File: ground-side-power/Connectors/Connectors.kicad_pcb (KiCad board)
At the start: 2 copper layers, 11 parts, among them J15 To Router, J16 To RLCS, J17 To DAQ Laptop, J18 Conn_01x02_Female, J19 Conn_01x02_Female, J20 To Ethernet, J21 To 5V M12, J22 To DAQ, J23 Extra M12, J24 Extra M12, J25 Extra M12

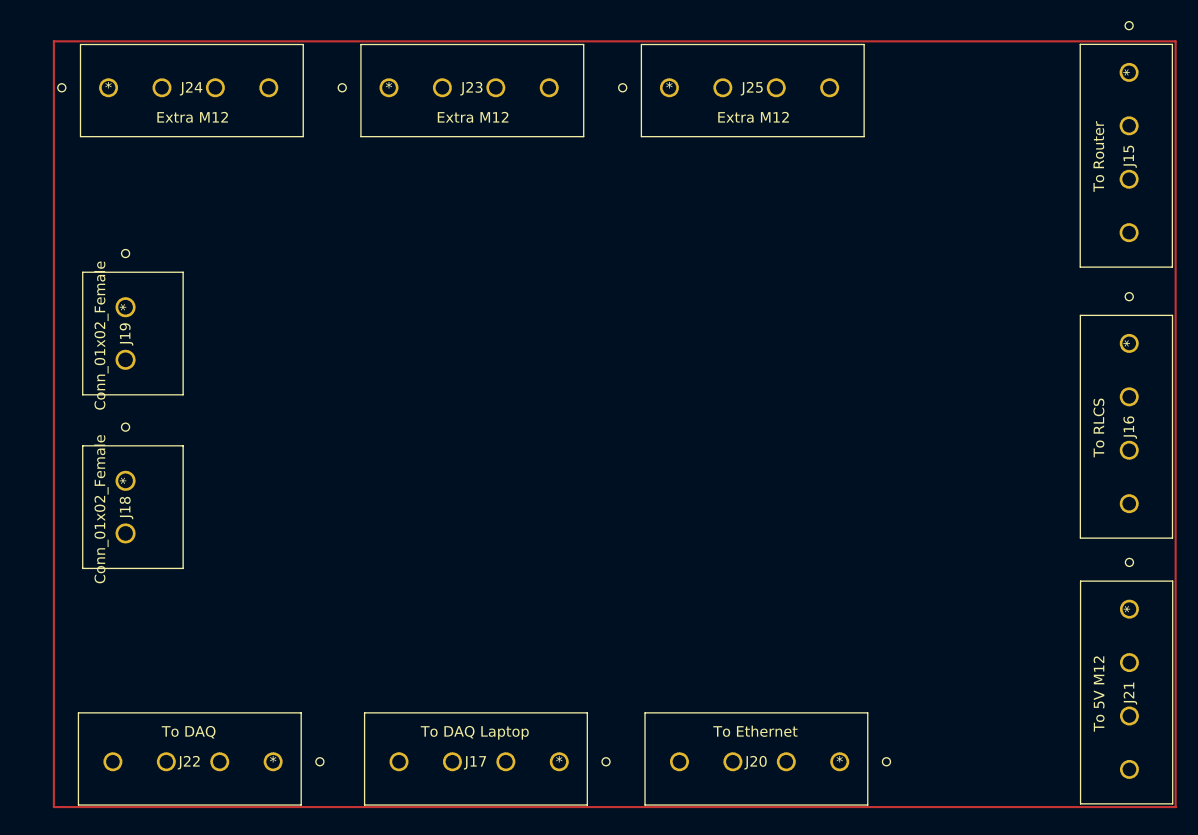
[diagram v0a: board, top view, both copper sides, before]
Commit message: PCB Layout First Draft
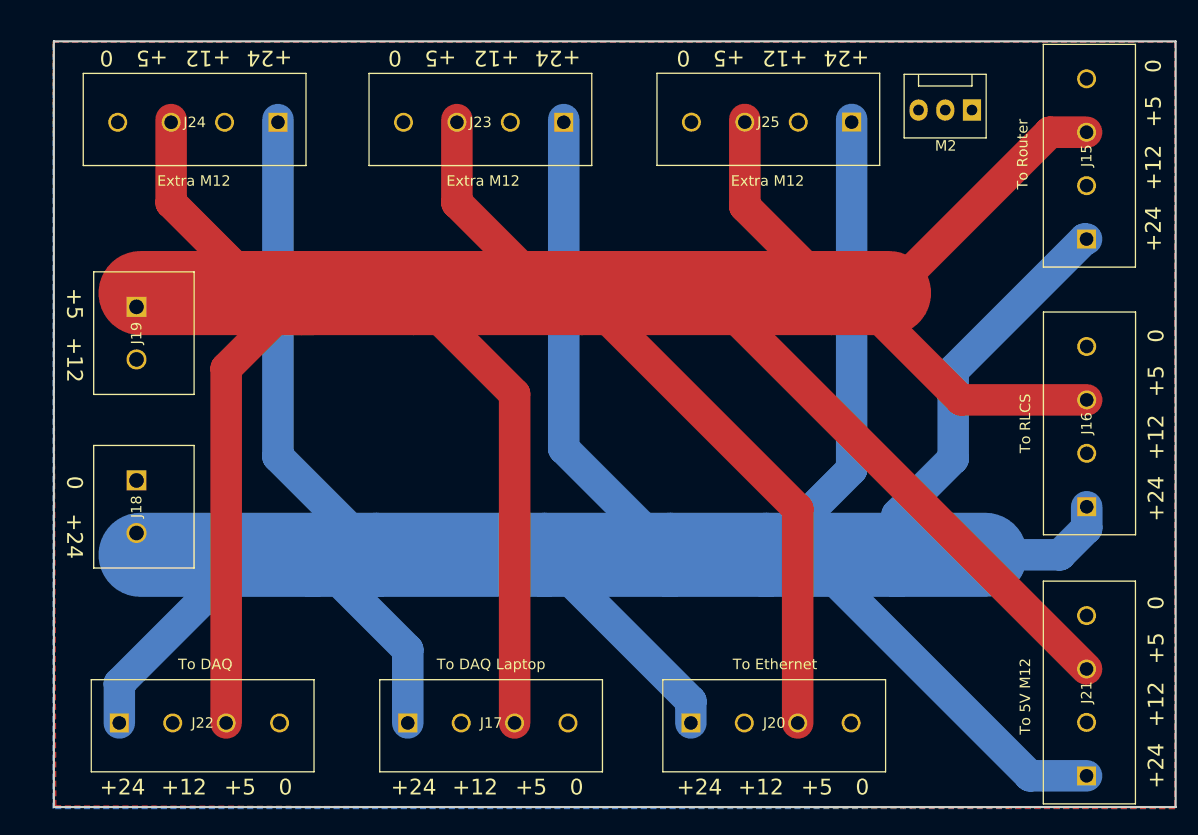
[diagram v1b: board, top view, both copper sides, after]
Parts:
- added M2: Fan_PC_Chassis, Connector:FanPinHeader_1x03_P2.54mm_Vertical, F.Cu at (178.6, 70.5)
- moved J25 17.6 mm to (167.1, 71.6), turned to 180 degrees
- moved J23 16.9 mm to (139.8, 71.6), turned to 180 degrees
- moved J24 16.4 mm to (112.6, 71.6), turned to 180 degrees
- moved J21 16.4 mm to (189.5, 133.8), turned to 90 degrees
- moved J15 16.4 mm to (189.5, 82.7), turned to 90 degrees
- moved J16 16.1 mm to (189.5, 108.2), turned to 90 degrees
- moved J22 15.1 mm to (97.5, 128.8), turned to 0 degrees
- moved J17 14.9 mm to (124.9, 128.8), turned to 0 degrees
- moved J20 14.6 mm to (151.8, 128.8), turned to 0 degrees
- moved J18 1.04 mm to (99.1, 105.7)
- moved J19 1.04 mm to (99.1, 89.2)
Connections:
- J15 pad 1: (no net) -> +24V
- J15 pad 2: (no net) -> +12V
- J15 pad 3: (no net) -> +5V
- J15 pad 4: (no net) -> GND
- J16 pad 1: (no net) -> +24V
- J16 pad 2: (no net) -> +12V
- J16 pad 3: (no net) -> +5V
- J16 pad 4: (no net) -> GND
- J17 pad 1: (no net) -> +24V
- J17 pad 2: (no net) -> +12V
- J17 pad 3: (no net) -> +5V
- J17 pad 4: (no net) -> GND
- J18 pad 1: (no net) -> GND
- J18 pad 2: (no net) -> +24V
- J19 pad 1: (no net) -> +5V
- J19 pad 2: (no net) -> +12V
- J20 pad 1: (no net) -> +24V
- J20 pad 2: (no net) -> +12V
- J20 pad 3: (no net) -> +5V
- J20 pad 4: (no net) -> GND
- J21 pad 1: (no net) -> +24V
- J21 pad 2: (no net) -> +12V
- J21 pad 3: (no net) -> +5V
- J21 pad 4: (no net) -> GND
- J22 pad 1: (no net) -> +24V
- J22 pad 2: (no net) -> +12V
- J22 pad 3: (no net) -> +5V
- J22 pad 4: (no net) -> GND
- J23 pad 1: (no net) -> +24V
- J23 pad 2: (no net) -> +12V
- J23 pad 3: (no net) -> +5V
- J23 pad 4: (no net) -> GND
- J24 pad 1: (no net) -> +24V
- J24 pad 2: (no net) -> +12V
- J24 pad 3: (no net) -> +5V
- J24 pad 4: (no net) -> GND
- J25 pad 1: (no net) -> +24V
- J25 pad 2: (no net) -> +12V
- J25 pad 3: (no net) -> +5V
- J25 pad 4: (no net) -> GND
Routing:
- net +5V: track 0.00 -> 380.6 mm
- net +24V: track 0.00 -> 364.0 mm
- added copper zone on B.Cu, net +12V
- added copper zone on F.Cu, net GND
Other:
- board outline added: 106.7 x 72.8 mm
- board text added: "+12"
- board text added: "+24"
- board text added: "+5"
- board text added: "0"

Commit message: Resolved Final Issues
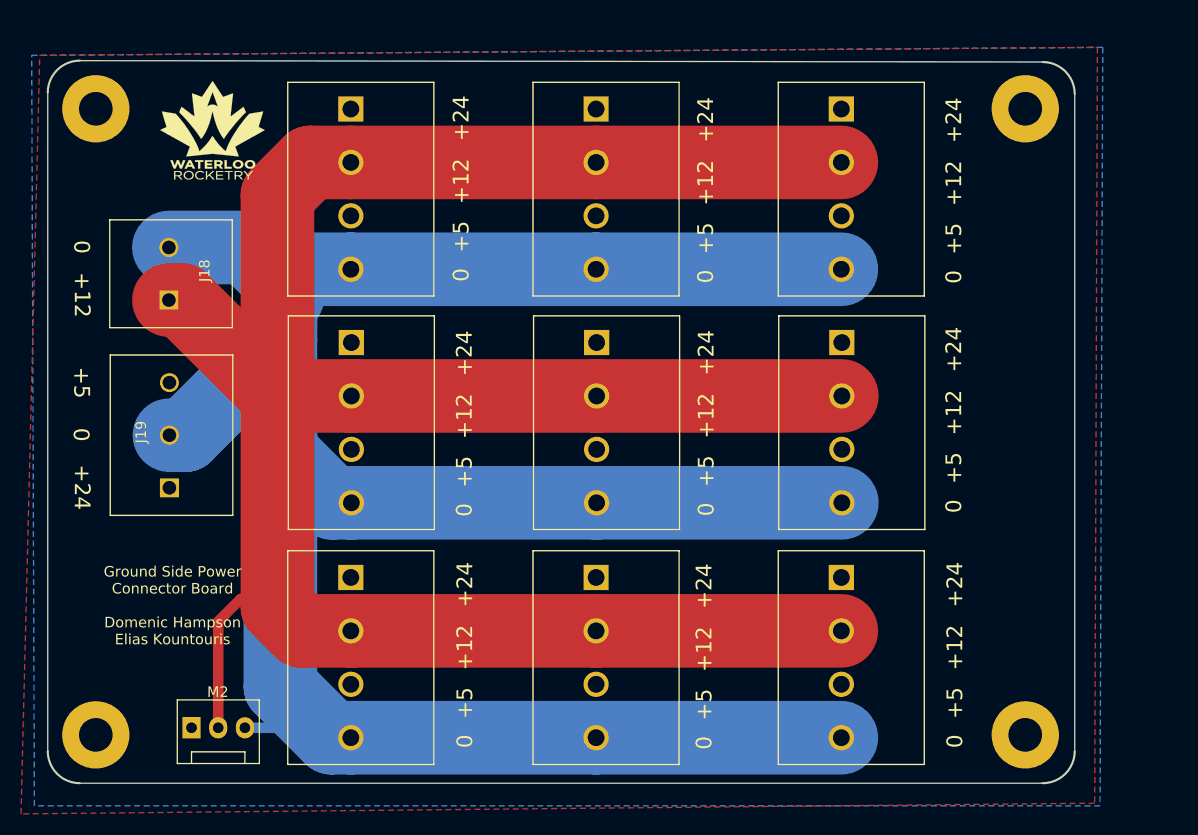
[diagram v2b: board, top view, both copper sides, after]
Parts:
- added ?: , , F.Cu at (95.2, 129.9)
- added ?: , , F.Cu at (183.6, 70.4)
- added ?: , , F.Cu at (183.6, 129.9)
- added G***: LOGO, rlcs:rocketry_logo_small, F.Cu at (106.3, 72.4)
- added REF**: MountingHole_3.2mm_M3_Pad, MountingHole:MountingHole_3.2mm_M3_Pad, F.Cu at (95.2, 70.4)
- J15, J16, J17, J20, J21, J22, J23, J24, J25: footprint GSP:EB21A-04-D -> GSP:CUI_TB008A-508-04BE
- J18: footprint GSP:OSTTA020161 -> GSP:1935310
- J19: footprint GSP:OSTTA020161 -> GSP:1935323
- moved M2 94.7 mm to (104.3, 129.2), turned to 0 degrees
- moved J25 64.4 mm to (119.5, 114.9), turned to -90 degrees
- moved J21 62.2 mm to (142.9, 92.6), turned to -90 degrees
- moved J20 59.1 mm to (142.8, 70.4), turned to -90 degrees
- moved J22 47.4 mm to (142.8, 114.9), turned to -90 degrees
- moved J17 43.5 mm to (166.2, 114.9), turned to -90 degrees
- moved J16 28.0 mm to (166.2, 92.6), turned to -90 degrees
- moved J15 26.4 mm to (166.2, 70.4), turned to -90 degrees
- moved J24 22.1 mm to (119.6, 92.6), turned to -90 degrees
- moved J23 20.3 mm to (119.5, 70.4), turned to -90 degrees
- moved J19 17.5 mm to (102.2, 106.4), turned to 90 degrees
- moved J18 17.4 mm to (102.2, 88.5), turned to 90 degrees
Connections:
- J18 pad 1: GND -> +12V
- J18 pad 2: +24V -> GND
- J19 pad 1: +5V -> +24V
- J19 pad 2: +12V -> GND
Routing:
- net +5V: track 380.6 -> 0.00 mm
- net +24V: track 364.0 -> 0.00 mm
- net GND: track 0.00 -> 244.5 mm
- net +12V: track 0.00 -> 233.1 mm
- added copper zone on F.Cu, net +24V
- added copper zone on B.Cu, net +5V
- removed copper zone on B.Cu, net +12V
- removed copper zone on F.Cu, net GND
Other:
- board size 106.7 x 72.8 mm -> 97.7 x 68.7 mm
- board text added: "Ground Side Power Connector Board Domenic Hampson Elias Kountouris"
